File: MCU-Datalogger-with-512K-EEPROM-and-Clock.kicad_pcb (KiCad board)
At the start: 2 copper layers, 54.5 x 36.5 mm, 30 parts, among them J1 Conn_01x04_Pin, J2 Conn_01x04_Pin, J3 Conn_01x09_Pin, J4 Conn_02x03_Odd_Even, U1 24LC1025, U2 24LC1025, U3 ATMEGA328P-AU, U4 DS1337S_, Y1 32.768 KHz, Y2 16 MHz

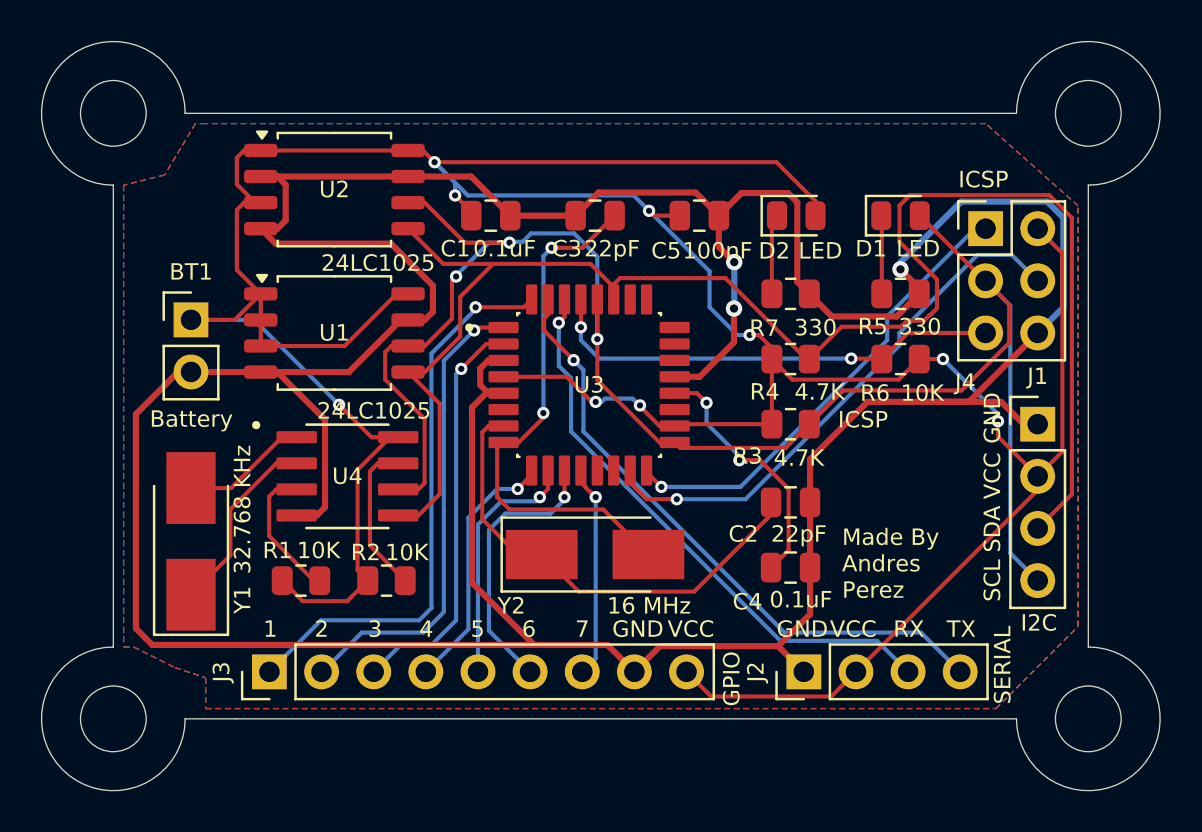
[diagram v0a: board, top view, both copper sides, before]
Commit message: 4layer board completed
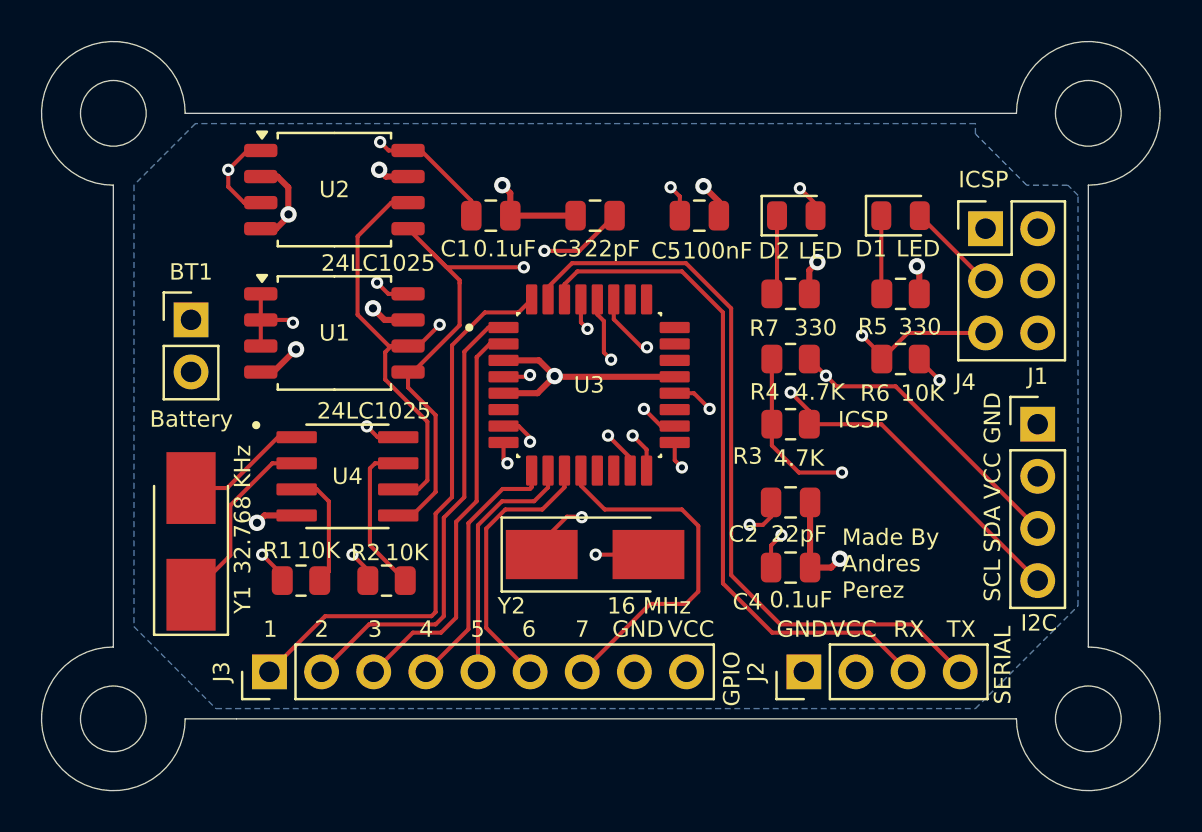
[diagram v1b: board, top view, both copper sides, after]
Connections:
- D1 pad 2: /SCL -> /SCK
- J4 pad 3: /SCL -> /SCK
- U3 pad 17: /SCL -> /SCK
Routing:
- net GND: track 200.2 -> 38.3 mm, vias 3 -> 11
- net /Vcc: track 176.9 -> 38.2 mm, vias 9 -> 13
- net /SCK: track 0.00 -> 24.6 mm, vias 0 -> 1
- net /SCL: track 83.8 -> 59.8 mm
- net /SDA: track 78.2 -> 58.0 mm, vias 0 -> 3
- net /D8: track 10.4 -> 17.7 mm, vias 1 -> 0
- net /TX: track 30.5 -> 37.0 mm, vias 1 -> 0
- net /RX: track 28.1 -> 33.5 mm, vias 1 -> 0
- net Net-(U3-PB6): track 23.1 -> 19.8 mm, vias 0 -> 3
- net /MOSI: track 26.6 -> 27.9 mm
- net Net-(U3-AREF): track 12.4 -> 11.4 mm
- net Net-(U4-~{INTA}): track 6.76 -> 5.86 mm
- net Net-(U3-PB7): track 26.0 -> 26.8 mm, vias 2 -> 3
- net /D3: track 23.0 -> 22.8 mm, vias 1 -> 0
- net /D5: track 12.5 -> 12.7 mm, vias 1 -> 0
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- added copper zone on In2.Cu, net /Vcc
- removed copper zone on F.Cu, net /Vcc
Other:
- copper layers 2 -> 4
